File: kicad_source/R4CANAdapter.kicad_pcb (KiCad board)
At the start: 2 copper layers, 48 x 52 mm, 33 parts, among them CN1 CONN_01X05, CN2 691322310004, CN3 GH_SM04B-GHS-TB, CN4 GH_SM04B-GHS-TB, CN5 SM04B-SRSS-TB, Q1 2N7002, Q2 2N7002, U1 TCAN332GDR, U2 24LC64

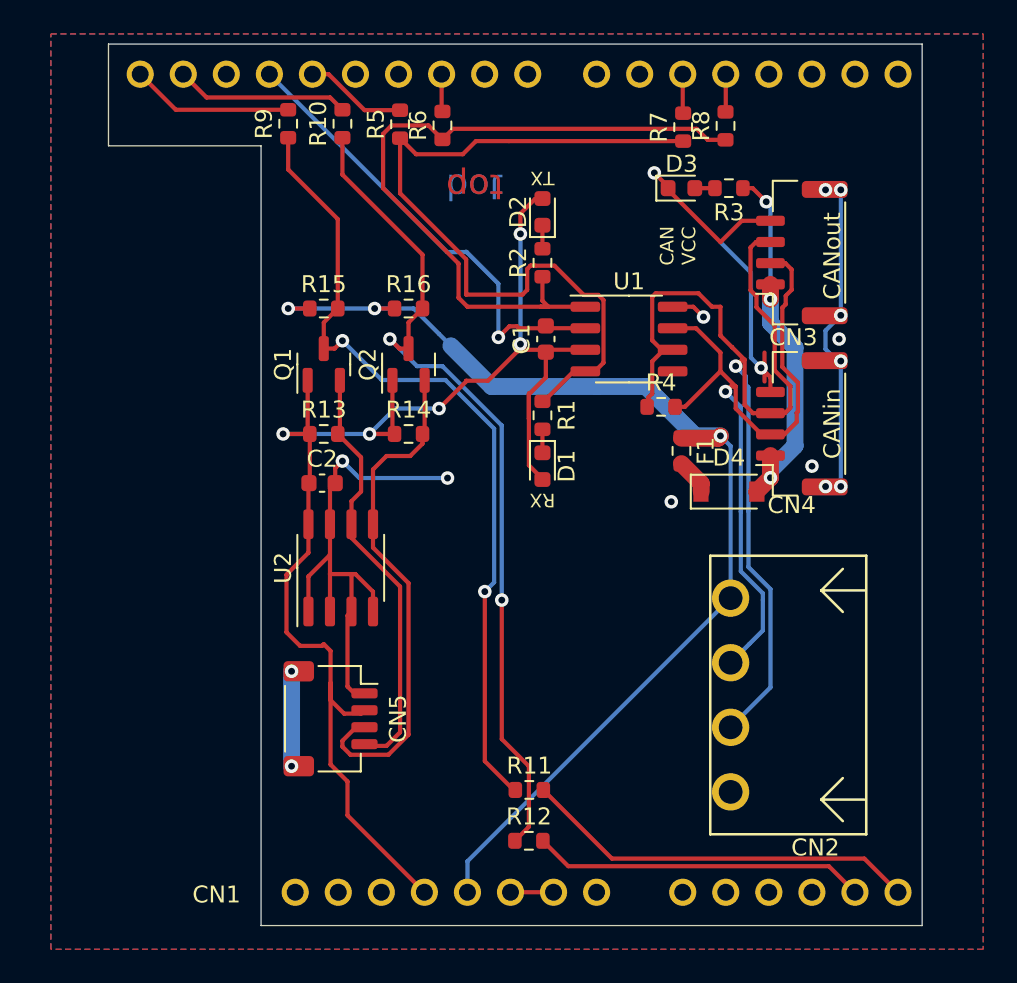
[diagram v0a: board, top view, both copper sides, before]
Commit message: beautified layout
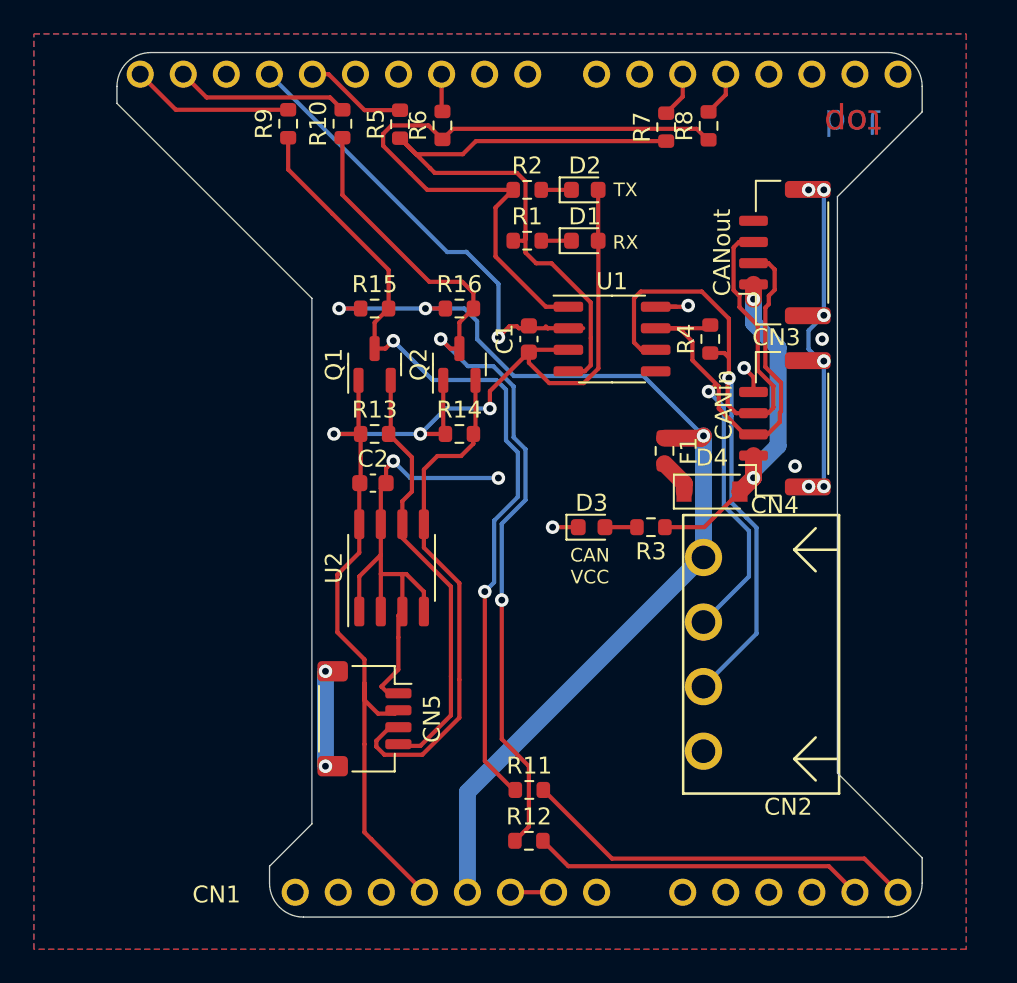
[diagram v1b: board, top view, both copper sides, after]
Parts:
- moved D3 20.7 mm to (145.5, 114.5)
- moved R3 20.5 mm to (149.0, 114.5)
- moved D1 13.5 mm to (145.1, 97.6), turned to 0 degrees
- moved R1 10.3 mm to (141.7, 97.6), turned to 0 degrees
- moved R4 4.94 mm to (152.5, 103.4), turned to 90 degrees
- moved R2 4.39 mm to (141.7, 94.6), turned to 0 degrees
- moved C2 3.00 mm to (132.6, 111.9)
- moved Q1 3.00 mm to (132.7, 104.9)
- moved Q2 3.00 mm to (137.7, 104.9)
- moved R13 3.00 mm to (132.7, 109.0)
- moved R14 3.00 mm to (137.7, 109.0)
- moved R15 3.00 mm to (132.7, 101.6)
- moved R16 3.00 mm to (137.7, 101.6)
- moved U2 3.00 mm to (133.7, 116.9)
- moved CN2 2.88 mm to (152.1, 122.0)
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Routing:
- net GND: track 84.6 -> 68.3 mm, vias 9 -> 8
- net +3V3: track 84.4 -> 75.5 mm, vias 5 -> 3
- net /CAN_RX: track 46.5 -> 40.5 mm
- net /CANL: track 56.7 -> 51.8 mm
- net /CAN_TX: track 42.8 -> 39.6 mm
- net +5V: track 67.0 -> 64.4 mm
- net /CANVCC: track 22.7 -> 20.4 mm, vias 3 -> 2
- net /CANH: track 44.7 -> 42.4 mm
- net /I2C_SDA: track 50.3 -> 52.6 mm
- net /I2C_SCL: track 48.7 -> 49.9 mm
- net Net-(D3-Pad2): track 1.30 -> 1.89 mm
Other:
- board size 48 x 52 mm -> 47.5 x 51 mm
